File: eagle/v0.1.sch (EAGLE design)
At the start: 12 parts, among them IC1 74LS595N

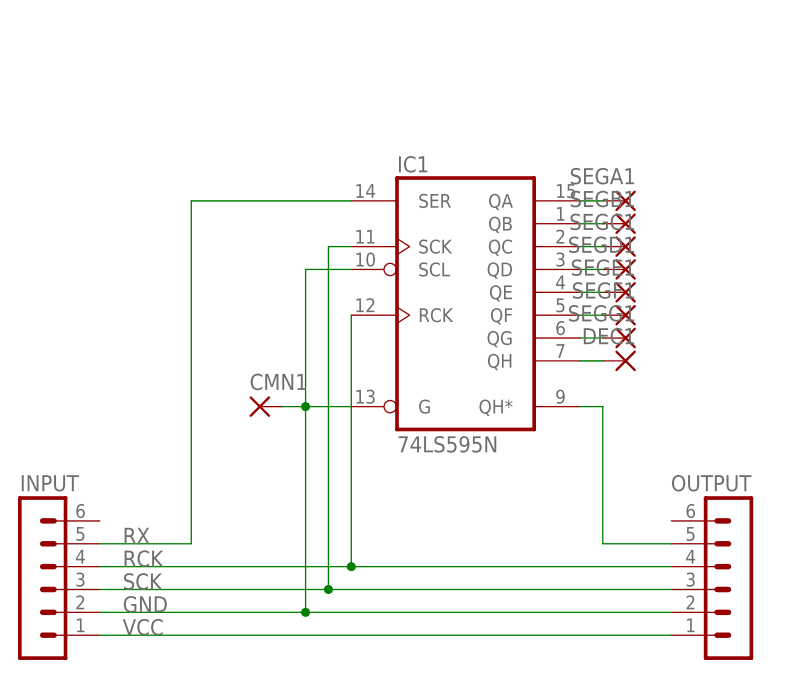
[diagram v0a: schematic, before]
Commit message: v0.1 as sent to fab
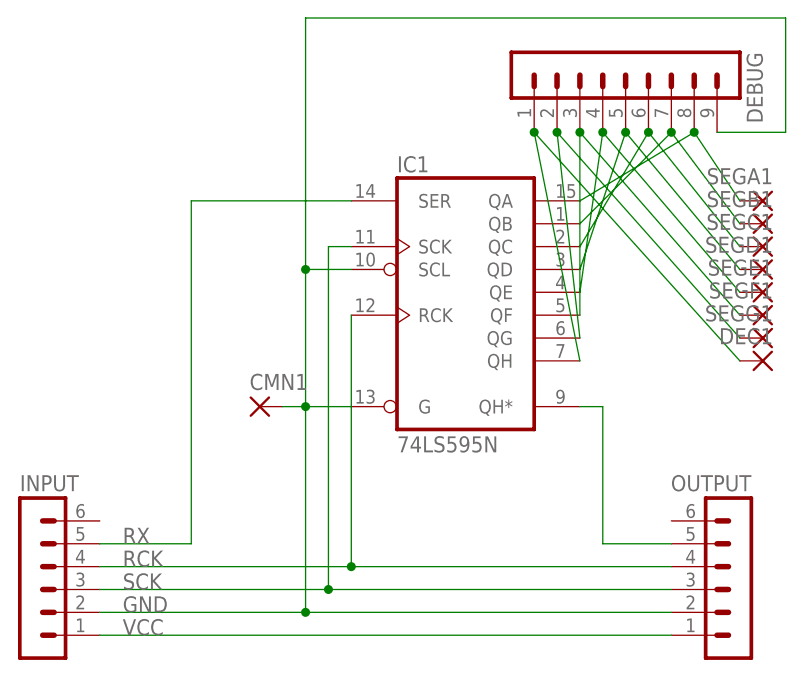
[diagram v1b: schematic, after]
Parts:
- added DEBUG: (no value), con-lstb:MA09-1
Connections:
- net GND: now also DEBUG.9
- net N$1: now also DEBUG.8
- net N$2: now also DEBUG.7
- net N$3: now also DEBUG.6
- net N$4: now also DEBUG.5
- net N$5: now also DEBUG.4
- net N$6: now also DEBUG.3
- net N$7: now also DEBUG.2
- net N$8: now also DEBUG.1
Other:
- moved on the sheet: DEC1, SEGA1, SEGB1, SEGC1, SEGD1, SEGE1, SEGF1, SEGG1
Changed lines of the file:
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@@
 <part name="INPUT" library="con-lstb" library_urn="urn:adsk.eagle:library:162" deviceset="MA06-1" device="" package3d_urn="urn:adsk.eagle:package:8340/1"/>
 <part name="OUTPUT" library="con-lstb" library_urn="urn:adsk.eagle:library:162" deviceset="MA06-1" device="" package3d_urn="urn:adsk.eagle:package:8340/1"/>
+<part name="DEBUG" library="con-lstb" library_urn="urn:adsk.eagle:library:162" deviceset="MA09-1" device="" package3d_urn="urn:adsk.eagle:package:8350/1"/>
 </parts>
 <sheets>
@@
 <attribute name="VALUE" x="14.097" y="19.558" size="1.778" layer="96"/>
 </instance>
-<instance part="DEC1" gate="P" x="55.88" y="27.94" smashed="yes" rot="MR0">
-<attribute name="NAME" x="57.023" y="29.7942" size="1.778" layer="95" rot="MR0"/>
-<attribute name="VALUE" x="57.023" y="24.638" size="1.778" layer="96" rot="MR0"/>
-</instance>
-<instance part="SEGB1" gate="P" x="55.88" y="43.18" smashed="yes" rot="MR0">
-<attribute name="NAME" x="57.023" y="45.0342" size="1.778" layer="95" rot="MR0"/>
-<attribute name="VALUE" x="57.023" y="39.878" size="1.778" layer="96" rot="MR0"/>
-</instance>
-<instance part="SEGC1" gate="P" x="55.88" y="40.64" smashed="yes" rot="MR0">
-<attribute name="NAME" x="57.023" y="42.4942" size="1.778" layer="95" rot="MR0"/>
-<attribute name="VALUE" x="57.023" y="37.338" size="1.778" layer="96" rot="MR0"/>
-</instance>
-<instance part="SEGA1" gate="P" x="55.88" y="45.72" smashed="yes" rot="MR0">
-<attribute name="NAME" x="57.023" y="47.5742" size="1.778" layer="95" rot="MR0"/>
-<attribute name="VALUE" x="57.023" y="42.418" size="1.778" layer="96" rot="MR0"/>
-</instance>
-<instance part="SEGF1" gate="P" x="55.88" y="33.02" smashed="yes" rot="MR0">
-<attribute name="NAME" x="57.023" y="34.8742" size="1.778" layer="95" rot="MR0"/>
-<attribute name="VALUE" x="57.023" y="29.718" size="1.778" layer="96" rot="MR0"/>
-</instance>
-<instance part="SEGG1" gate="P" x="55.88" y="30.48" smashed="yes" rot="MR0">
-<attribute name="NAME" x="57.023" y="32.3342" size="1.778" layer="95" rot="MR0"/>
-<attribute name="VALUE" x="57.023" y="27.178" size="1.778" layer="96" rot="MR0"/>
-</instance>
-<instance part="SEGD1" gate="P" x="55.88" y="38.1" smashed="yes" rot="MR0">
-<attribute name="NAME" x="57.023" y="39.9542" size="1.778" layer="95" rot="MR0"/>
-<attribute name="VALUE" x="57.023" y="34.798" size="1.778" layer="96" rot="MR0"/>
-</instance>
-<instance part="SEGE1" gate="P" x="55.88" y="35.56" smashed="yes" rot="MR0">
-<attribute name="NAME" x="57.023" y="37.4142" size="1.778" layer="95" rot="MR0"/>
-<attribute name="VALUE" x="57.023" y="32.258" size="1.778" layer="96" rot="MR0"/>
+<instance part="DEC1" gate="P" x="71.12" y="27.94" smashed="yes" rot="MR0">
+<attribute name="NAME" x="72.263" y="29.7942" size="1.778" layer="95" rot="MR0"/>
+<attribute name="VALUE" x="72.263" y="24.638" size="1.778" layer="96" rot="MR0"/>
+</instance>
+<instance part="SEGB1" gate="P" x="71.12" y="43.18" smashed="yes" rot="MR0">
+<attribute name="NAME" x="72.263" y="45.0342" size="1.778" layer="95" rot="MR0"/>
+<attribute name="VALUE" x="72.263" y="39.878" size="1.778" layer="96" rot="MR0"/>
+</instance>
+<instance part="SEGC1" gate="P" x="71.12" y="40.64" smashed="yes" rot="MR0">
+<attribute name="NAME" x="72.263" y="42.4942" size="1.778" layer="95" rot="MR0"/>
+<attribute name="VALUE" x="72.263" y="37.338" size="1.778" layer="96" rot="MR0"/>
+</instance>
+<instance part="SEGA1" gate="P" x="71.12" y="45.72" smashed="yes" rot="MR0">
+<attribute name="NAME" x="72.263" y="47.5742" size="1.778" layer="95" rot="MR0"/>
+<attribute name="VALUE" x="72.263" y="42.418" size="1.778" layer="96" rot="MR0"/>
+</instance>
+<instance part="SEGF1" gate="P" x="71.12" y="33.02" smashed="yes" rot="MR0">
+<attribute name="NAME" x="72.263" y="34.8742" size="1.778" layer="95" rot="MR0"/>
+<attribute name="VALUE" x="72.263" y="29.718" size="1.778" layer="96" rot="MR0"/>
+</instance>
+<instance part="SEGG1" gate="P" x="71.12" y="30.48" smashed="yes" rot="MR0">
+<attribute name="NAME" x="72.263" y="32.3342" size="1.778" layer="95" rot="MR0"/>
+<attribute name="VALUE" x="72.263" y="27.178" size="1.778" layer="96" rot="MR0"/>
+</instance>
+<instance part="SEGD1" gate="P" x="71.12" y="38.1" smashed="yes" rot="MR0">
+<attribute name="NAME" x="72.263" y="39.9542" size="1.778" layer="95" rot="MR0"/>
+<attribute name="VALUE" x="72.263" y="34.798" size="1.778" layer="96" rot="MR0"/>
+</instance>
+<instance part="SEGE1" gate="P" x="71.12" y="35.56" smashed="yes" rot="MR0">
+<attribute name="NAME" x="72.263" y="37.4142" size="1.778" layer="95" rot="MR0"/>
+<attribute name="VALUE" x="72.263" y="32.258" size="1.778" layer="96" rot="MR0"/>
 </instance>
 <instance part="IC1" gate="A" x="38.1" y="35.56" smashed="yes">
@@
 <attribute name="VALUE" x="69.85" y="-7.62" size="1.778" layer="96" rot="MR0"/>
 <attribute name="NAME" x="69.85" y="13.462" size="1.778" layer="95" rot="MR0"/>
+</instance>
+<instance part="DEBUG" gate="1" x="55.88" y="60.96" smashed="yes" rot="R270">
+<attribute name="VALUE" x="40.64" y="62.23" size="1.778" layer="96" rot="R270"/>
+<attribute name="NAME" x="69.342" y="62.23" size="1.778" layer="95" rot="R270"/>
 </instance>
 </instances>
@@
 <pinref part="IC1" gate="A" pin="QA"/>
 <pinref part="SEGA1" gate="P" pin="P"/>
-<wire x1="50.8" y1="45.72" x2="53.34" y2="45.72" width="0.1524" layer="91"/>
+<wire x1="50.8" y1="45.72" x2="63.5" y2="53.34" width="0.1524" layer="91"/>
+<pinref part="DEBUG" gate="1" pin="8"/>
+<wire x1="63.5" y1="53.34" x2="68.58" y2="45.72" width="0.1524" layer="91"/>
+<junction x="63.5" y="53.34"/>
 </segment>
 </net>
@@
 <pinref part="IC1" gate="A" pin="QB"/>
 <pinref part="SEGB1" gate="P" pin="P"/>
-<wire x1="50.8" y1="43.18" x2="53.34" y2="43.18" width="0.1524" layer="91"/>
+<wire x1="50.8" y1="43.18" x2="60.96" y2="53.34" width="0.1524" layer="91"/>
+<pinref part="DEBUG" gate="1" pin="7"/>
+<wire x1="60.96" y1="53.34" x2="68.58" y2="43.18" width="0.1524" layer="91"/>
+<junction x="60.96" y="53.34"/>
 </segment>
 </net>
@@
 <pinref part="IC1" gate="A" pin="QC"/>
 <pinref part="SEGC1" gate="P" pin="P"/>
-<wire x1="50.8" y1="40.64" x2="53.34" y2="40.64" width="0.1524" layer="91"/>
+<wire x1="50.8" y1="40.64" x2="58.42" y2="53.34" width="0.1524" layer="91"/>
+<pinref part="DEBUG" gate="1" pin="6"/>
+<wire x1="58.42" y1="53.34" x2="68.58" y2="40.64" width="0.1524" layer="91"/>
+<junction x="58.42" y="53.34"/>
 </segment>
 </net>
@@
 <pinref part="IC1" gate="A" pin="QD"/>
 <pinref part="SEGD1" gate="P" pin="P"/>
-<wire x1="50.8" y1="38.1" x2="53.34" y2="38.1" width="0.1524" layer="91"/>
+<wire x1="50.8" y1="38.1" x2="55.88" y2="53.34" width="0.1524" layer="91"/>
+<pinref part="DEBUG" gate="1" pin="5"/>
+<wire x1="55.88" y1="53.34" x2="68.58" y2="38.1" width="0.1524" layer="91"/>
+<junction x="55.88" y="53.34"/>
 </segment>
 </net>
@@
 <pinref part="IC1" gate="A" pin="QE"/>
 <pinref part="SEGE1" gate="P" pin="P"/>
-<wire x1="50.8" y1="35.56" x2="53.34" y2="35.56" width="0.1524" layer="91"/>
+<wire x1="50.8" y1="35.56" x2="53.34" y2="53.34" width="0.1524" layer="91"/>
+<pinref part="DEBUG" gate="1" pin="4"/>
+<wire x1="53.34" y1="53.34" x2="68.58" y2="35.56" width="0.1524" layer="91"/>
+<junction x="53.34" y="53.34"/>
 </segment>
 </net>
@@
 <pinref part="IC1" gate="A" pin="QF"/>
 <pinref part="SEGF1" gate="P" pin="P"/>
-<wire x1="50.8" y1="33.02" x2="53.34" y2="33.02" width="0.1524" layer="91"/>
+<wire x1="50.8" y1="33.02" x2="50.8" y2="53.34" width="0.1524" layer="91"/>
+<pinref part="DEBUG" gate="1" pin="3"/>
+<wire x1="50.8" y1="53.34" x2="68.58" y2="33.02" width="0.1524" layer="91"/>
+<junction x="50.8" y="53.34"/>
 </segment>
 </net>
@@
 <pinref part="IC1" gate="A" pin="QG"/>
 <pinref part="SEGG1" gate="P" pin="P"/>
-<wire x1="50.8" y1="30.48" x2="53.34" y2="30.48" width="0.1524" layer="91"/>
+<wire x1="50.8" y1="30.48" x2="48.26" y2="53.34" width="0.1524" layer="91"/>
+<pinref part="DEBUG" gate="1" pin="2"/>
+<wire x1="48.26" y1="53.34" x2="68.58" y2="30.48" width="0.1524" layer="91"/>
+<junction x="48.26" y="53.34"/>
 </segment>
 </net>
@@
 <wire x1="20.32" y1="38.1" x2="20.32" y2="22.86" width="0.1524" layer="91"/>
 <pinref part="OUTPUT" gate="1" pin="2"/>
+<wire x1="20.32" y1="38.1" x2="20.32" y2="66.04" width="0.1524" layer="91"/>
+<junction x="20.32" y="38.1"/>
+<wire x1="20.32" y1="66.04" x2="73.66" y2="66.04" width="0.1524" layer="91"/>
+<wire x1="73.66" y1="66.04" x2="73.66" y2="53.34" width="0.1524" layer="91"/>
+<pinref part="DEBUG" gate="1" pin="9"/>
+<wire x1="73.66" y1="53.34" x2="66.04" y2="53.34" width="0.1524" layer="91"/>
 </segment>
 </net>
@@
 <pinref part="IC1" gate="A" pin="QH"/>
 <pinref part="DEC1" gate="P" pin="P"/>
-<wire x1="50.8" y1="27.94" x2="53.34" y2="27.94" width="0.1524" layer="91"/>
-</segment>
-</net>
+<wire x1="50.8" y1="27.94" x2="45.72" y2="53.34" width="0.1524" layer="91"/>
+<pinref part="DEBUG" gate="1" pin="1"/>
+<wire x1="45.72" y1="53.34" x2="68.58" y2="27.94" width="0.1524" layer="91"/>
+<junction x="45.72" y="53.34"/>
+</segment>
+</net>
